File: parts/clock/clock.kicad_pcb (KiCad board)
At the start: 2 copper layers, 50 x 77 mm, 32 parts, among them J1 ~{CLK}, J2 CLK, J3 HLT, J4 PWR, SW1 SW_Push, SW2 SW_SPDT, U1 LM555, U2 LM555, U3 LM555, U4 74HC04, U5 74HC08, U6 74HC32

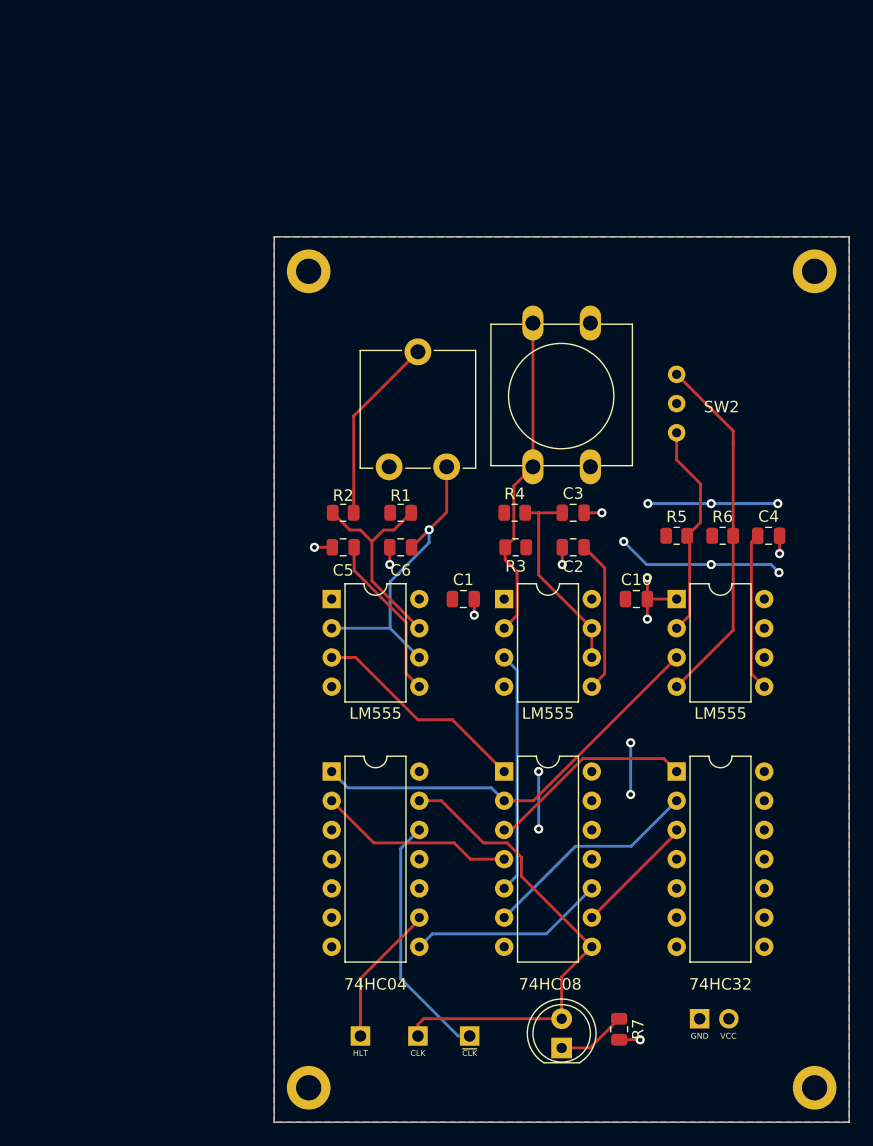
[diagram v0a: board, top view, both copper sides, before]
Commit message: SMD Clock
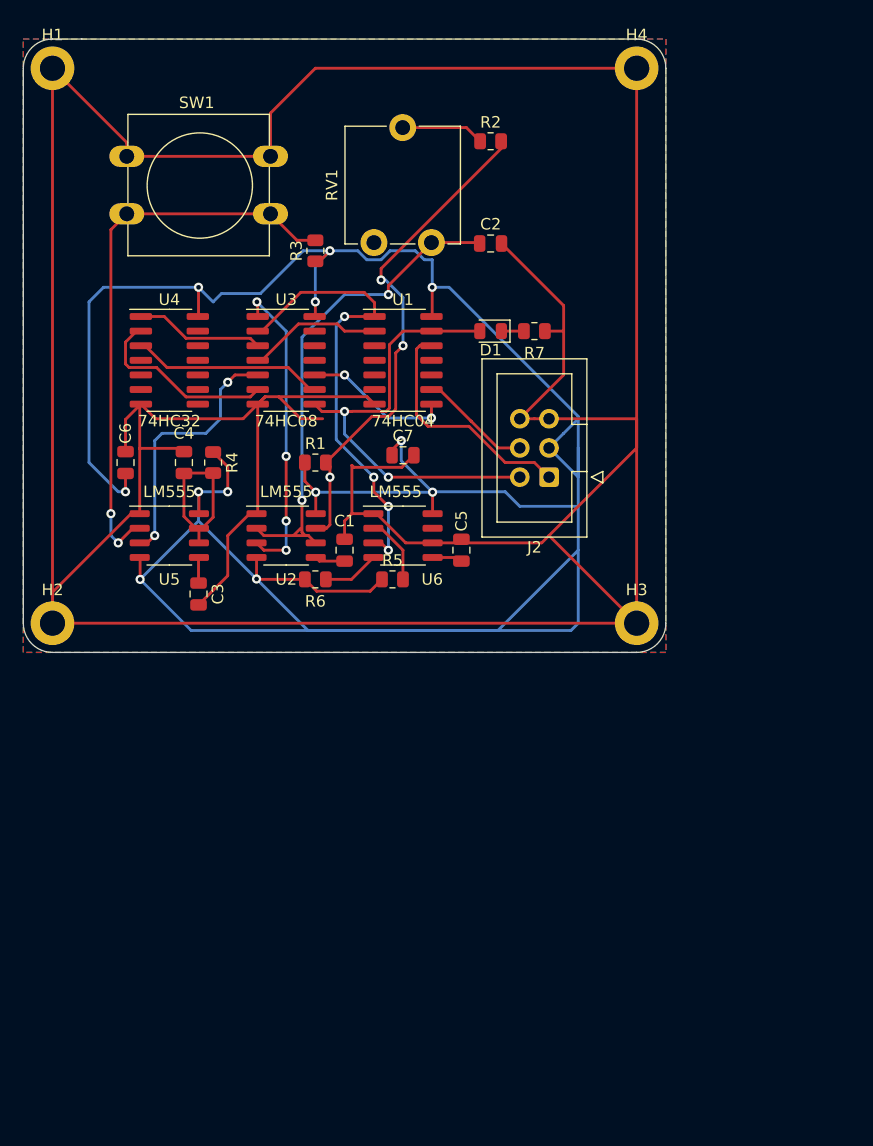
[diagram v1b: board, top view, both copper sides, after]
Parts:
- removed C10: 0.1µF, Capacitor_SMD:C_0805_2012Metric
- removed J1: ~{CLK}, Connector_PinHeader_2.54mm:PinHeader_1x01_P2.54mm_Vertical
- removed J3: HLT, Connector_PinHeader_2.54mm:PinHeader_1x01_P2.54mm_Vertical
- removed J4: PWR, Connector_PinHeader_2.54mm:PinHeader_1x02_P2.54mm_Vertical
- removed SW2: SW_SPDT, clock:switch
- added C7: 0.1µF, Capacitor_SMD:C_0805_2012Metric, F.Cu at (76.2, 87.0)
- C1, C3: value 0.1µF -> 0.01µF
- C2: value 0.01µF -> 1µF
- C4: value 0.01µF -> 0.1µF
- C6: value 1µF -> 0.1µF
- D1: footprint LED_THT:LED_D5.0mm -> LED_SMD:LED_0805_2012Metric
- J2: value CLK -> Conn_01x08; footprint Connector_PinHeader_2.54mm:PinHeader_1x01_P2.54mm_Vertical -> Connector_IDC:IDC-Header_2x03_P2.54mm_Vertical; moved to F.Cu
- U1: value LM555 -> 74HC04; footprint Package_DIP:DIP-8_W7.62mm -> Package_SO:SO-14_3.9x8.65mm_P1.27mm
- U2: footprint Package_DIP:DIP-8_W7.62mm -> Package_SO:SO-8_3.9x4.9mm_P1.27mm
- U3: value LM555 -> 74HC08; footprint Package_DIP:DIP-8_W7.62mm -> Package_SO:SO-14_3.9x8.65mm_P1.27mm
- U4: value 74HC04 -> 74HC32; footprint Package_DIP:DIP-14_W7.62mm -> Package_SO:SO-14_3.9x8.65mm_P1.27mm
- U5: value 74HC08 -> LM555; footprint Package_DIP:DIP-14_W7.62mm -> Package_SO:SO-8_3.9x4.9mm_P1.27mm
- U6: value 74HC32 -> LM555; footprint Package_DIP:DIP-14_W7.62mm -> Package_SO:SO-8_3.9x4.9mm_P1.27mm
- moved H4 90.0 mm to (96.5, 53.3)
- moved D1 62.6 mm to (83.8, 76.2), turned to 180 degrees
- moved R7 61.2 mm to (87.6, 76.2), turned to 0 degrees
- moved C4 51.2 mm to (57.1, 87.6), turned to 90 degrees
- moved J2 49.9 mm to (88.9, 88.9)
- moved H2 46.1 mm to (45.7, 101.6)
- moved SW1 42.8 mm to (52.2, 61.0), turned to 0 degrees
- moved U3 39.8 mm to (66.0, 78.7)
- moved U4 38.4 mm to (55.9, 78.7)
- moved U5 35.6 mm to (55.9, 94.0)
- moved R6 35.6 mm to (68.6, 97.8)
- moved R2 34.8 mm to (83.8, 59.7), turned to 0 degrees
- moved H3 34.3 mm to (96.5, 101.6)
- moved C3 33.3 mm to (58.4, 99.1), turned to -90 degrees
- moved U6 31.4 mm to (76.2, 94.0)
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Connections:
- C1 pad 1: VCC -> Net-(C1-Pad1)
- C6 pad 1: Net-(C6-Pad1) -> VCC
- J2 pad 1: /CLK -> /~{CLK}
- R4 pad 2: Net-(C3-Pad1) -> Net-(C4-Pad1)
- RV1 pad 1: Net-(C6-Pad1) -> Net-(C2-Pad1)
- U1 pad 1: GND -> Net-(U1-Pad1)
- U1 pad 2: Net-(C6-Pad1) -> Net-(U1-Pad2)
- U1 pad 3: Net-(U1-Pad3) -> unconnected-(U1-Pad3)
- U1 pad 4: VCC -> unconnected-(U1-Pad4)
- U1 pad 5: Net-(C5-Pad1) -> unconnected-(U1-Pad5)
- U1 pad 6: Net-(C6-Pad1) -> unconnected-(U1-Pad6)
- U1 pad 7: Net-(R1-Pad2) -> GND
- U1 pad 8: VCC -> /~{HLT}
- U2 pad 2: Net-(R3-Pad2) -> Net-(C2-Pad1)
- U2 pad 5: Net-(C2-Pad1) -> Net-(C1-Pad1)
- U2 pad 6: Net-(C3-Pad1) -> Net-(C2-Pad1)
- U2 pad 7: Net-(C3-Pad1) -> Net-(R1-Pad2)
- U3 pad 1: GND -> Net-(U2-Pad3)
- U3 pad 2: Net-(R5-Pad2) -> Net-(U1-Pad1)
- U3 pad 4: Net-(R6-Pad2) -> Net-(U1-Pad2)
- U3 pad 5: Net-(C4-Pad1) -> Net-(U3-Pad5)
- U3 pad 6: GND -> Net-(U3-Pad6)
- U3 pad 7: unconnected-(U3-Pad7) -> GND
- U3 pad 8: VCC -> /CLK
- U4 pad 12: /~{CLK} -> unconnected-(U4-Pad12)
- U4 pad 13: /CLK -> unconnected-(U4-Pad13)
- U4 pad 2: Net-(U4-Pad2) -> Net-(U3-Pad6)
- U4 pad 3: unconnected-(U4-Pad3) -> Net-(U3-Pad9)
- U4 pad 8: /~{HLT} -> unconnected-(U4-Pad8)
- U4 pad 9: /HLT -> unconnected-(U4-Pad9)
- U5 pad 1: Net-(U1-Pad3) -> GND
- U5 pad 2: Net-(U3-Pad3) -> Net-(R3-Pad2)
- U5 pad 3: Net-(U5-Pad3) -> Net-(U3-Pad5)
- U5 pad 4: Net-(U4-Pad2) -> VCC
- U5 pad 5: Net-(U2-Pad3) -> Net-(C3-Pad1)
- U5 pad 6: Net-(U5-Pad6) -> Net-(C4-Pad1)
- U5 pad 7: GND -> Net-(C4-Pad1)
- U5 pad 8: /CLK -> VCC
- U6 pad 1: Net-(U5-Pad3) -> GND
- U6 pad 2: Net-(U5-Pad6) -> Net-(R5-Pad2)
- U6 pad 3: Net-(U5-Pad9) -> Net-(U1-Pad1)
- U6 pad 4: unconnected-(U6-Pad4) -> Net-(R6-Pad2)
- U6 pad 5: unconnected-(U6-Pad5) -> Net-(C5-Pad1)
- U6 pad 6: unconnected-(U6-Pad6) -> GND
- U6 pad 7: GND -> unconnected-(U6-Pad7)
- U6 pad 8: unconnected-(U6-Pad8) -> VCC
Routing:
- net GND: track 17.0 -> 372.1 mm, vias 9 -> 0
- net VCC: track 35.4 -> 265.1 mm, vias 10 -> 12
- net Net-(U1-Pad1): track 0.00 -> 39.8 mm, vias 0 -> 4
- net Net-(C2-Pad1): track 13.3 -> 43.5 mm, vias 0 -> 2
- net Net-(C6-Pad1): track 26.9 -> 0.00 mm, vias 1 -> 0
- net Net-(R6-Pad2): track 31.2 -> 4.92 mm
- net Net-(R1-Pad2): track 18.1 -> 43.8 mm, vias 0 -> 3
- net Net-(U3-Pad3): track 36.2 -> 11.2 mm
- net Net-(U3-Pad5): track 0.00 -> 22.6 mm, vias 0 -> 2
- net Net-(R3-Pad2): track 28.4 -> 49.2 mm, vias 0 -> 2
- net Net-(U5-Pad6): track 19.2 -> 0.00 mm
- net Net-(U1-Pad3): track 19.1 -> 0.00 mm
- net Net-(U5-Pad3): track 18.0 -> 0.00 mm
- net Net-(U4-Pad2): track 17.1 -> 0.00 mm
- net Net-(U3-Pad9): track 0.00 -> 16.7 mm
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- added copper zone on F.Cu, net GND
- added copper zone on B.Cu, net VCC
- removed copper zone on B.Cu, net GND
- removed copper zone on F.Cu, net VCC
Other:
- board size 50 x 77 mm -> 55.9 x 53.3 mm
- board text removed: "GND"
- board text removed: "VCC"
